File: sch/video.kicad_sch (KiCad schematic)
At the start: 14 parts

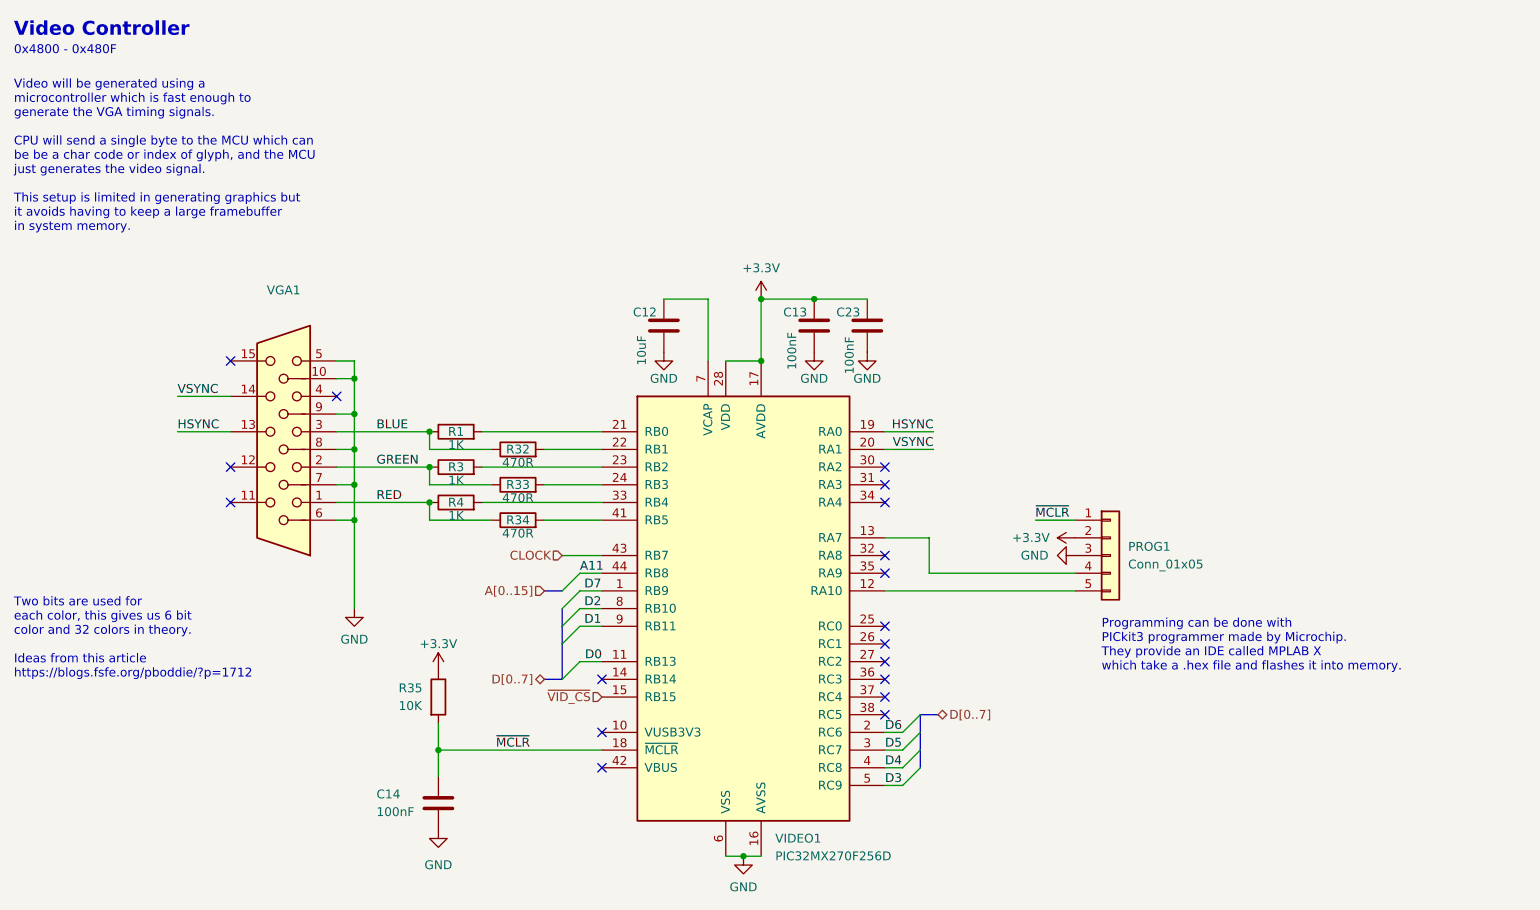
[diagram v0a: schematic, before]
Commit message: improve routing
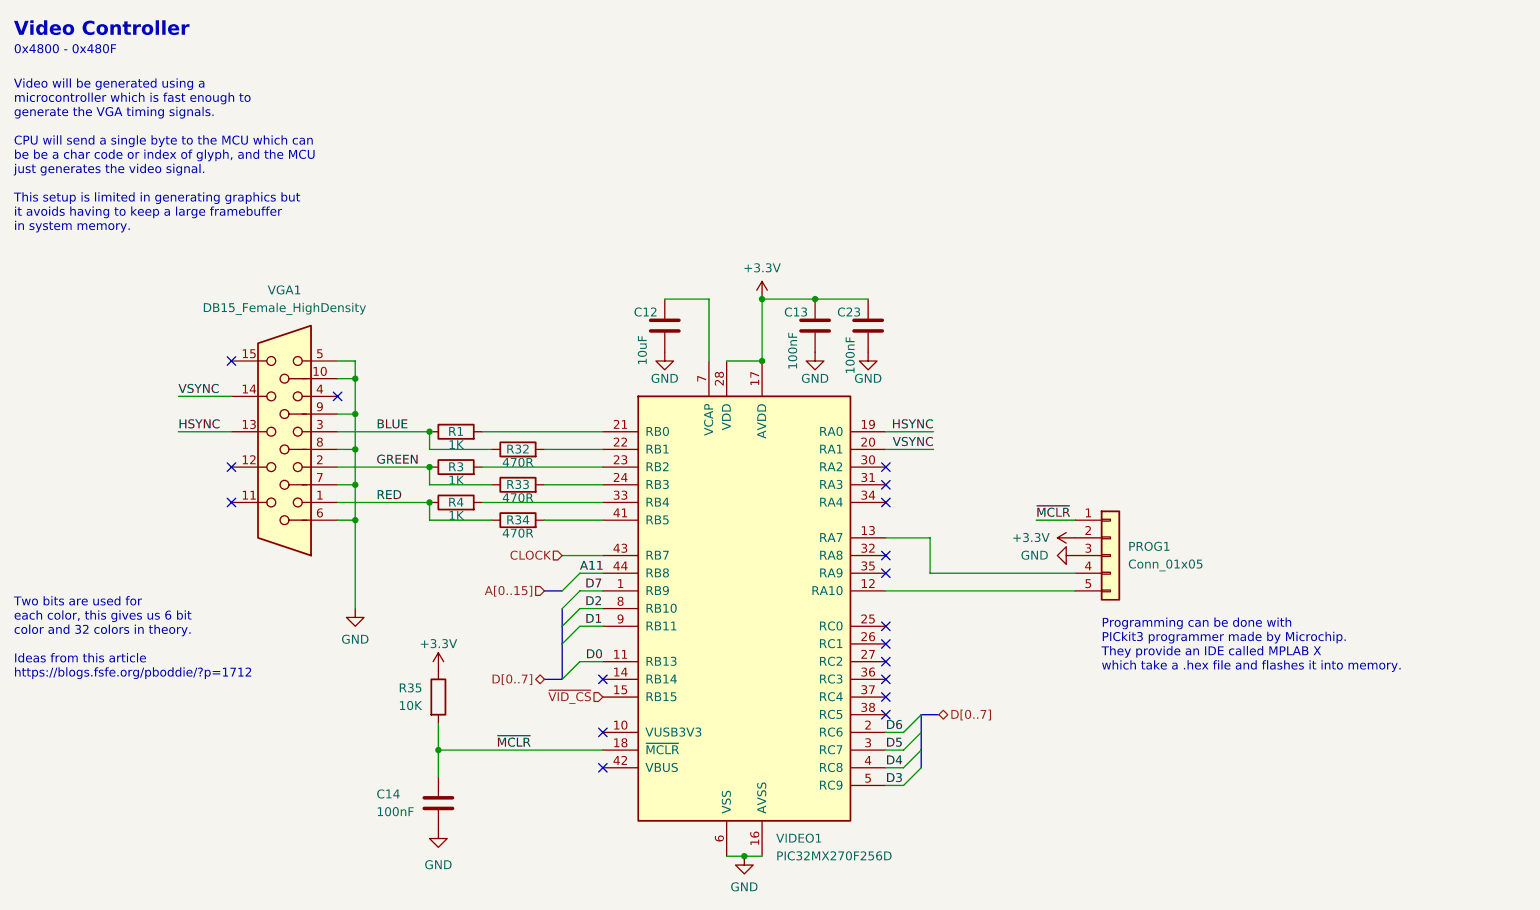
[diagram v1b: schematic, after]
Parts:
- VGA1: value (none) -> DB15_Female_HighDensity; footprint (none) -> Connector_Dsub:DSUB-15-HD_Female_Horizontal_P2.29x1.98mm_EdgePinOffset3.03mm_Housed_MountingHolesOffset4.94mm
